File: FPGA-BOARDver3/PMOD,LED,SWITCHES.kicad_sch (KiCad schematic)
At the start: 86 parts, among them P1 PMOD-Device-x2-Type-Generic-A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, P2 PMOD-Device-x2-Type-Generic-A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, Q1 BC107, Q2 BC107, Q3 BC107, Q4 BC107, Q5 BC107, Q6 BC107, SW2 SW_Push, SW3 SW_Push, SW4 SW_Push, SW5 SW_Push, SW6 SW_SP3T, SW7 SW_SP3T

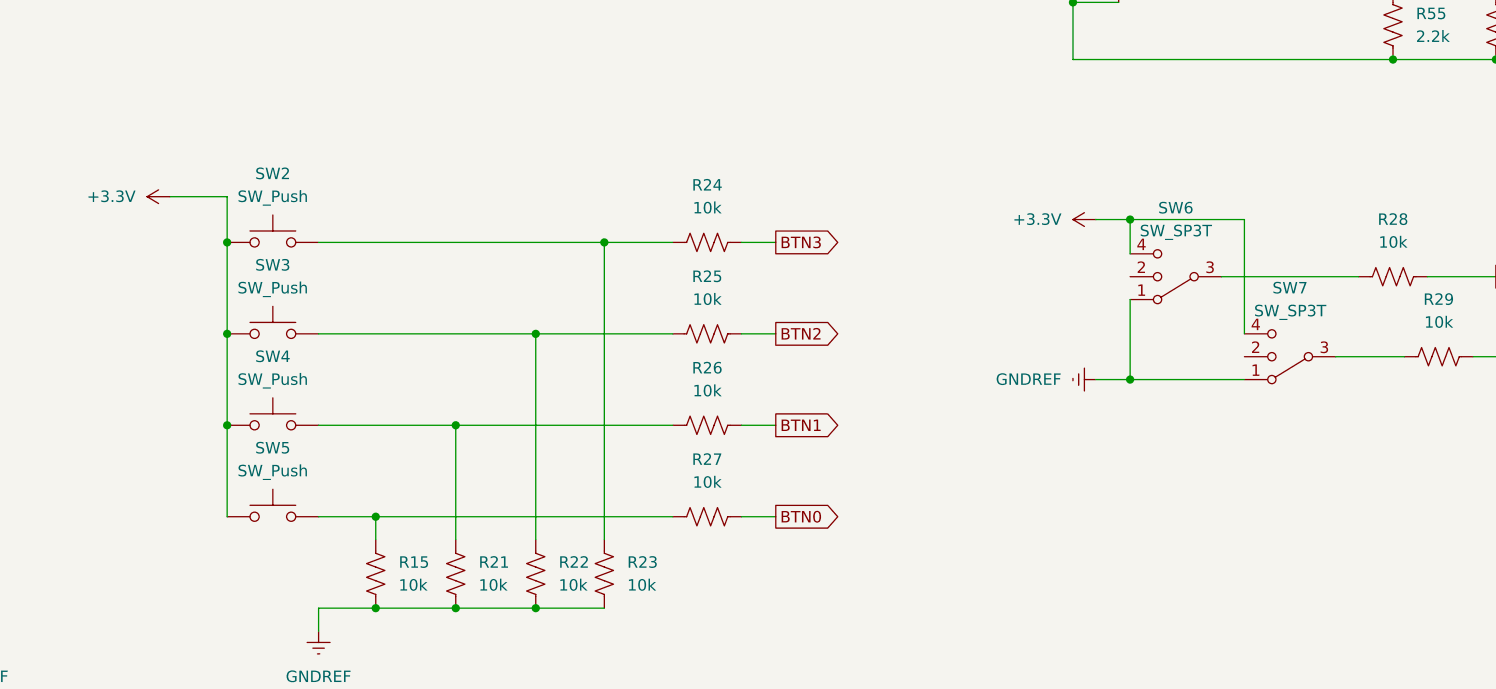
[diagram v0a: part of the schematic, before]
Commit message: spdif fpga bansks
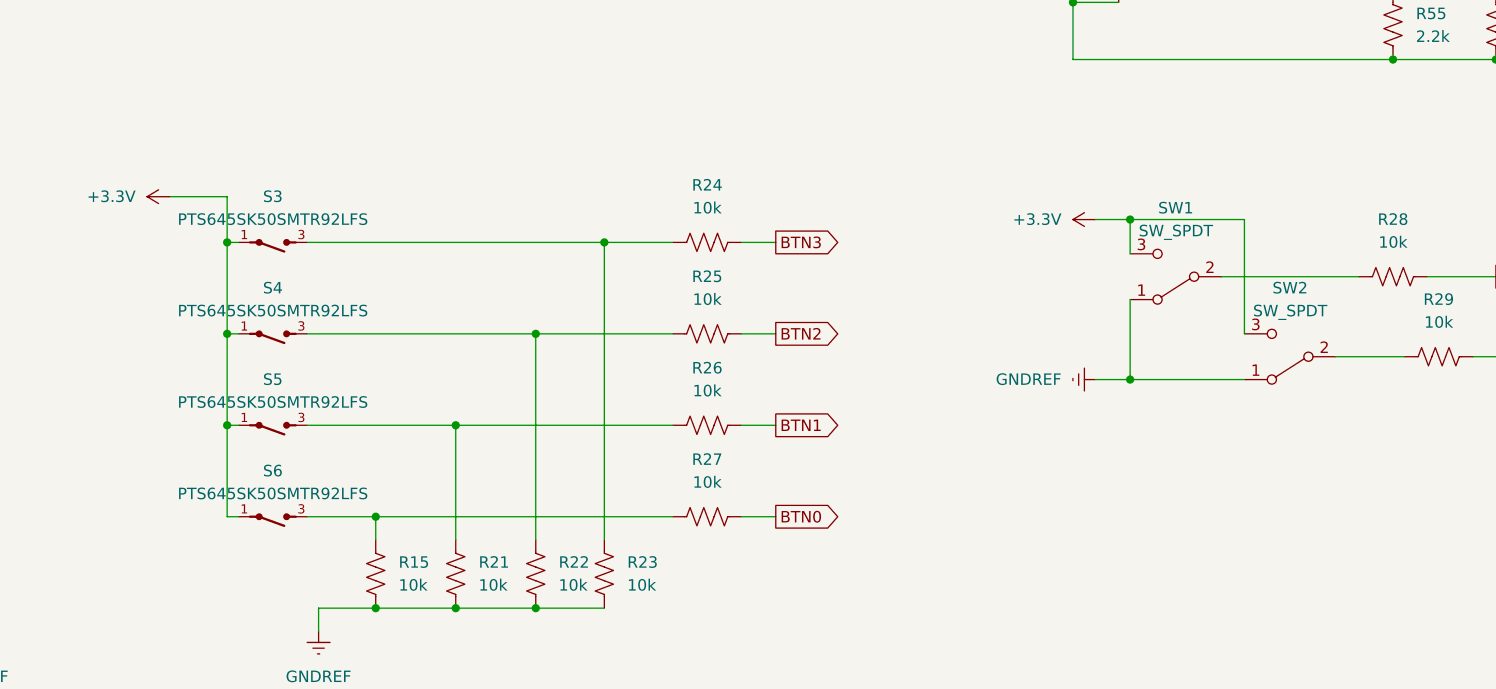
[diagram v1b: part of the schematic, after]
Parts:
- removed SW2, SW3, SW4, SW5: SW_Push, symbol Switch:SW_Push
- removed SW6, SW7: SW_SP3T, symbol Switch2:SW_SP3T
- added S3, S4, S5, S6: PTS645SK50SMTR92LFS, footprints:SW_PTS645SK50SMTR92LFS, symbol PTS645SK50SMTR92LFS:PTS645SK50SMTR92LFS
- added SW1, SW2: SW_SPDT, footprints:SS-12D10G5_XKB, symbol Switch2:SW_SPDT
- P1, P2: footprint pmod-conn_6x2:pmod_pin_array_6x2 -> footprints:CONN_PPPC062LJBN-RC_SUL
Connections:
- net +3.3V: now also S3.1, S4.1, S5.1, S6.1, SW1.3 (C), SW2.3 (C)
- net GNDREF: now also SW1.1 (A), SW2.1 (A)
- net at R15.1, R27.1: now also S6.3
- net at R21.1, R26.1: now also S5.3
- net at R22.1, R25.1: now also S4.3
- net at R29.1: now also SW2.2 (B)
- net at R23.1, R24.1: now also S3.3
- net at R28.1: now also SW1.2 (B)
